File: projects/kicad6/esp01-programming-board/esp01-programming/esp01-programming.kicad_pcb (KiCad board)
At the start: 2 copper layers, 113.8 x 39.6 mm, 20 parts, among them J1 Conn_01x06_Female, J2 Conn_01x05_Female, SW1 SW_DIP_x01, SW2 SW_DIP_x01, U1 AMS1117-3.3, U2 ESP01

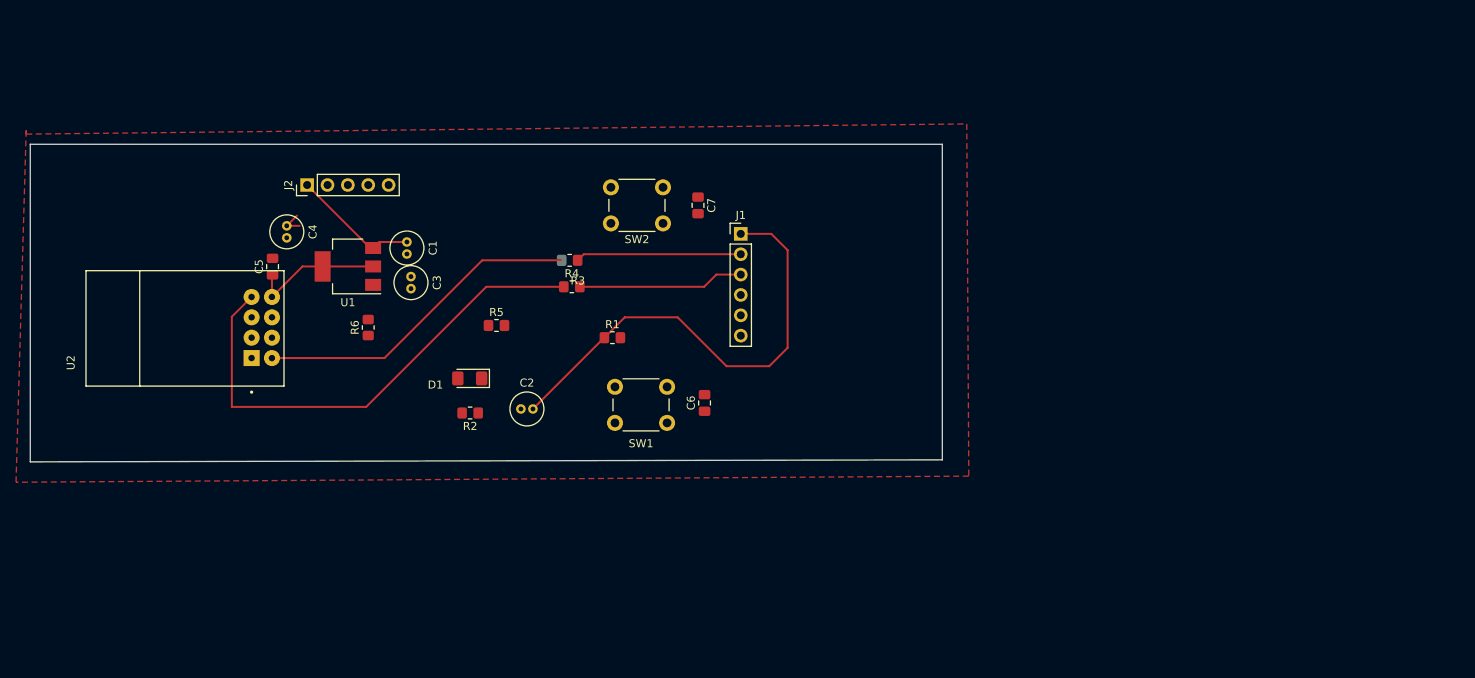
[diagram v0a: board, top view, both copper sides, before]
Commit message: Add new changes
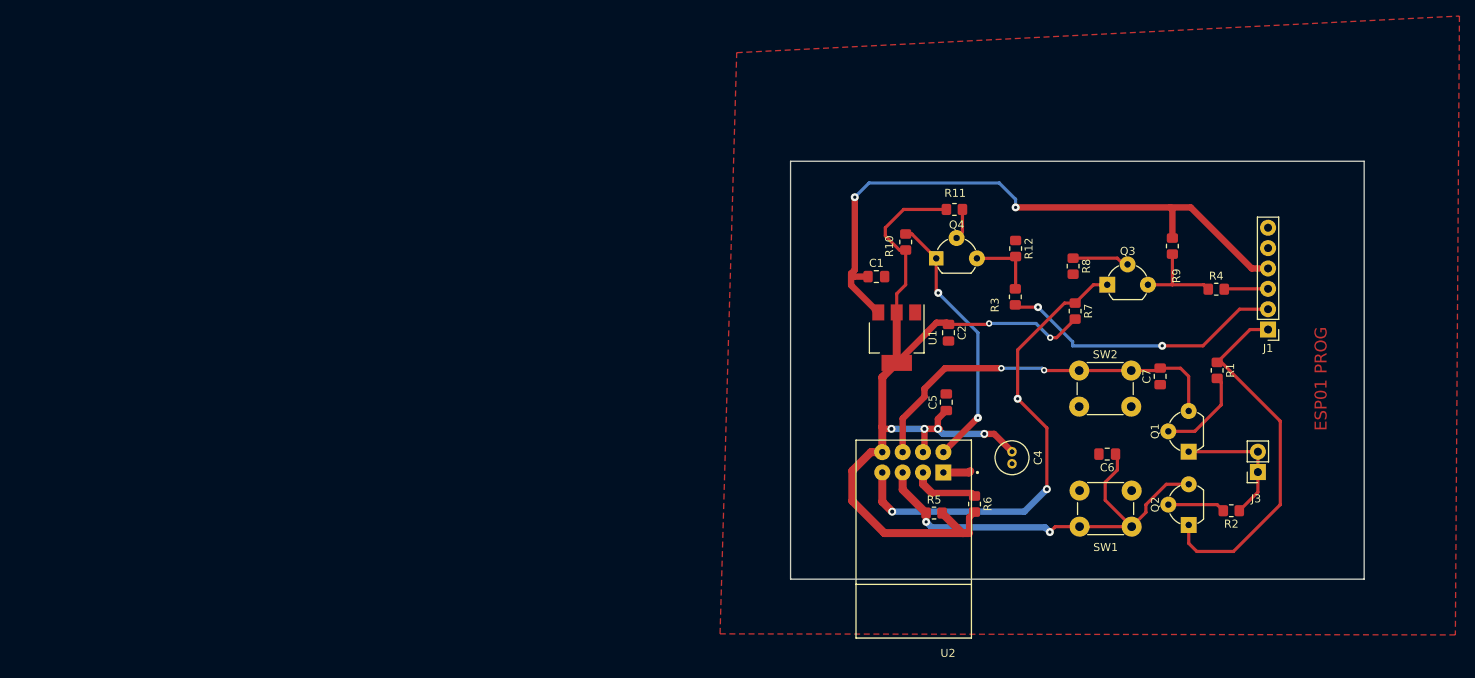
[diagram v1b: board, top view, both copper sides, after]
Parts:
- removed C3: 220u, Capacitor_THT:C_Radial_D4.0mm_H7.0mm_P1.50mm
- removed D1: D, Diode_SMD:D_1206_3216Metric_Pad1.42x1.75mm_HandSolder
- removed J2: Conn_01x05_Female, Connector_PinHeader_2.54mm:PinHeader_1x05_P2.54mm_Vertical
- added J3: RTS pinout, MY_ETCHING:PinSocket_1x02_P2.54mm_Vertical_ETCH, F.Cu at (169.4, 114.6)
- added Q1: 2N3904, Package_TO_SOT_THT:TO-92_Wide, F.Cu at (160.8, 112.0)
- added Q2: 2N3904, Package_TO_SOT_THT:TO-92_Wide, F.Cu at (160.8, 121.2)
- added Q3: 2N3904, Package_TO_SOT_THT:TO-92_Wide, F.Cu at (150.6, 91.2)
- added Q4: 2N3904, Package_TO_SOT_THT:TO-92_Wide, F.Cu at (129.3, 87.9)
- added R10: 10k, Resistor_SMD:R_0805_2012Metric_Pad1.20x1.40mm_HandSolder, F.Cu at (125.5, 85.9)
- added R11: 10k, Resistor_SMD:R_0805_2012Metric_Pad1.20x1.40mm_HandSolder, F.Cu at (131.6, 81.8)
- added R12: 10k, Resistor_SMD:R_0805_2012Metric_Pad1.20x1.40mm_HandSolder, F.Cu at (139.2, 86.7)
- added R7: 10k, Resistor_SMD:R_0805_2012Metric_Pad1.20x1.40mm_HandSolder, F.Cu at (146.6, 94.5)
- added R8: 10k, Resistor_SMD:R_0805_2012Metric_Pad1.20x1.40mm_HandSolder, F.Cu at (146.4, 88.9)
- added R9: 10k, Resistor_SMD:R_0805_2012Metric_Pad1.20x1.40mm_HandSolder, F.Cu at (158.8, 86.4)
- C1: value 100u -> 10u; footprint Capacitor_THT:C_Radial_D4.0mm_H7.0mm_P1.50mm -> Capacitor_SMD:C_0805_2012Metric_Pad1.18x1.45mm_HandSolder
- C2: value 2.2u -> 47u; footprint Capacitor_THT:C_Radial_D4.0mm_H7.0mm_P1.50mm -> Capacitor_SMD:C_0805_2012Metric_Pad1.18x1.45mm_HandSolder
- J1: value Conn_01x06_Female -> FT232RL header
- R1: value 680 -> 10k
- moved R2 95.7 mm to (166.1, 119.4)
- moved C4 94.8 mm to (138.7, 112.0)
- moved U2 94.6 mm to (126.4, 122.9), turned to 180 degrees
- moved C5 85.7 mm to (130.5, 105.8)
- moved R4 80.4 mm to (164.2, 91.7)
- moved R6 78.8 mm to (134.1, 118.5), turned to -90 degrees
- moved R1 75.6 mm to (164.3, 101.9), turned to -90 degrees
- moved U1 69.1 mm to (124.4, 97.8), turned to -90 degrees
- moved J1 66.9 mm to (170.7, 96.8), turned to 180 degrees
- moved C7 61.5 mm to (157.2, 102.6), turned to 90 degrees
- moved R5 59.4 mm to (129.0, 119.7)
- moved SW1 59.4 mm to (153.7, 121.4)
- moved C1 58.7 mm to (121.8, 90.2), turned to 0 degrees
- moved R3 55.8 mm to (139.2, 92.7), turned to 90 degrees
- moved SW2 55.1 mm to (147.1, 101.9), turned to 0 degrees
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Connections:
- C1 pad 1: 5v -> +5V
- C2 pad 1: uC_RST -> 3.3v
- C2 pad 2: DTR -> GND
- J1 pad 4: unconnected-(J1-Pad4) -> +5V
- R1 pad 2: GND -> Net-(Q1-Pad2)
- R2 pad 1: 3.3v -> RTS
- R2 pad 2: uC_RST -> Net-(Q2-Pad2)
- R3 pad 2: uC_TX -> ft_RX
- R4 pad 1: uC_RX -> ft_TX
- U1 pad 3: 5v -> +5V
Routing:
- net 3.3v: track 20.4 -> 120.4 mm, vias 0 -> 6
- net +5V: track 0.00 -> 80.2 mm, vias 0 -> 2
- net PRG: track 0.00 -> 54.8 mm, vias 0 -> 2
- net uC_RST: track 0.00 -> 48.1 mm, vias 0 -> 2
- net RTS: track 0.00 -> 17.0 mm
- net 5v: track 16.0 -> 0.00 mm
- net Net-(J1-Pad2): track 20.7 -> 36.1 mm, vias 0 -> 2
- net Net-(J1-Pad3): track 20.7 -> 5.49 mm
- net DTR: track 58.9 -> 46.0 mm
- net Net-(Q1-Pad2): track 0.00 -> 11.7 mm
- net ft_TX: track 0.00 -> 11.6 mm
- net ft_RX: track 0.00 -> 8.97 mm
- net Net-(R6-Pad1): track 0.00 -> 8.50 mm
- net uC_TX: track 41.2 -> 33.2 mm, vias 0 -> 2
- net Net-(Q2-Pad2): track 0.00 -> 7.17 mm
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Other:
- board size 113.8 x 39.6 mm -> 71.6 x 52.1 mm
- board text added: "ESP01 PROG"
